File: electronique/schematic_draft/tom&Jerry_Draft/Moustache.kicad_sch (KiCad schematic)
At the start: 9 parts, among them IC3 IIM-20670, J4 Conn_01x08, J5 Conn_01x04, J6 Conn_01x04, J7 Conn_01x04, J8 Conn_01x04

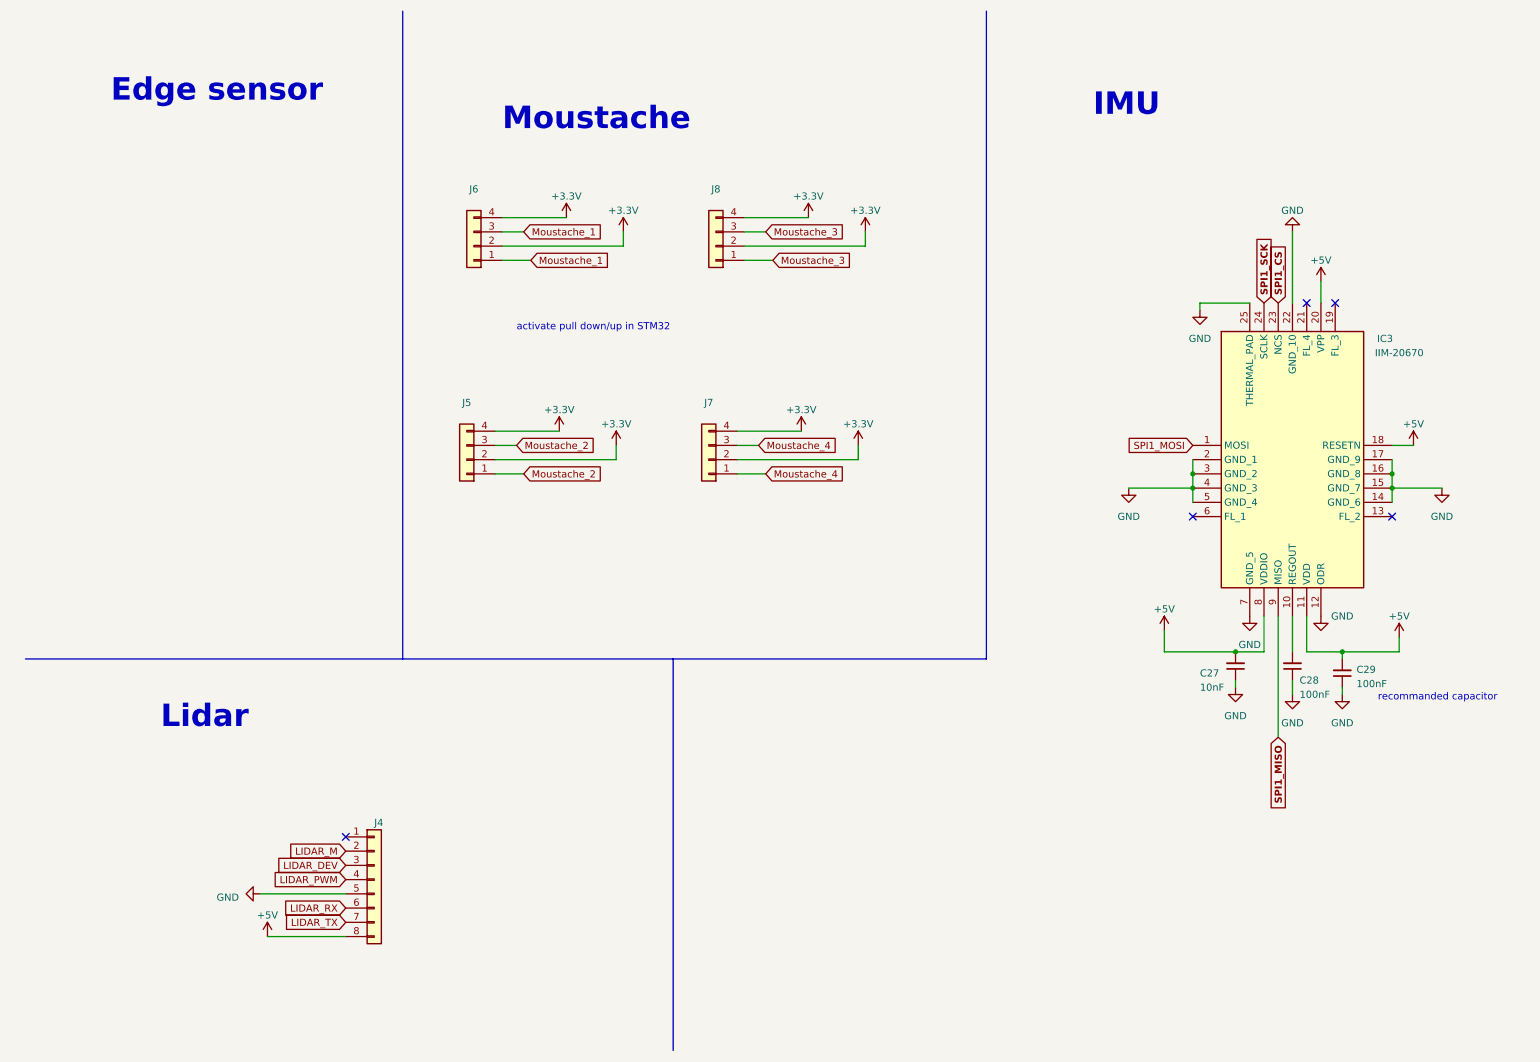
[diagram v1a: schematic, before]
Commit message: STM32 KiCAD V2 - 18.09.2024
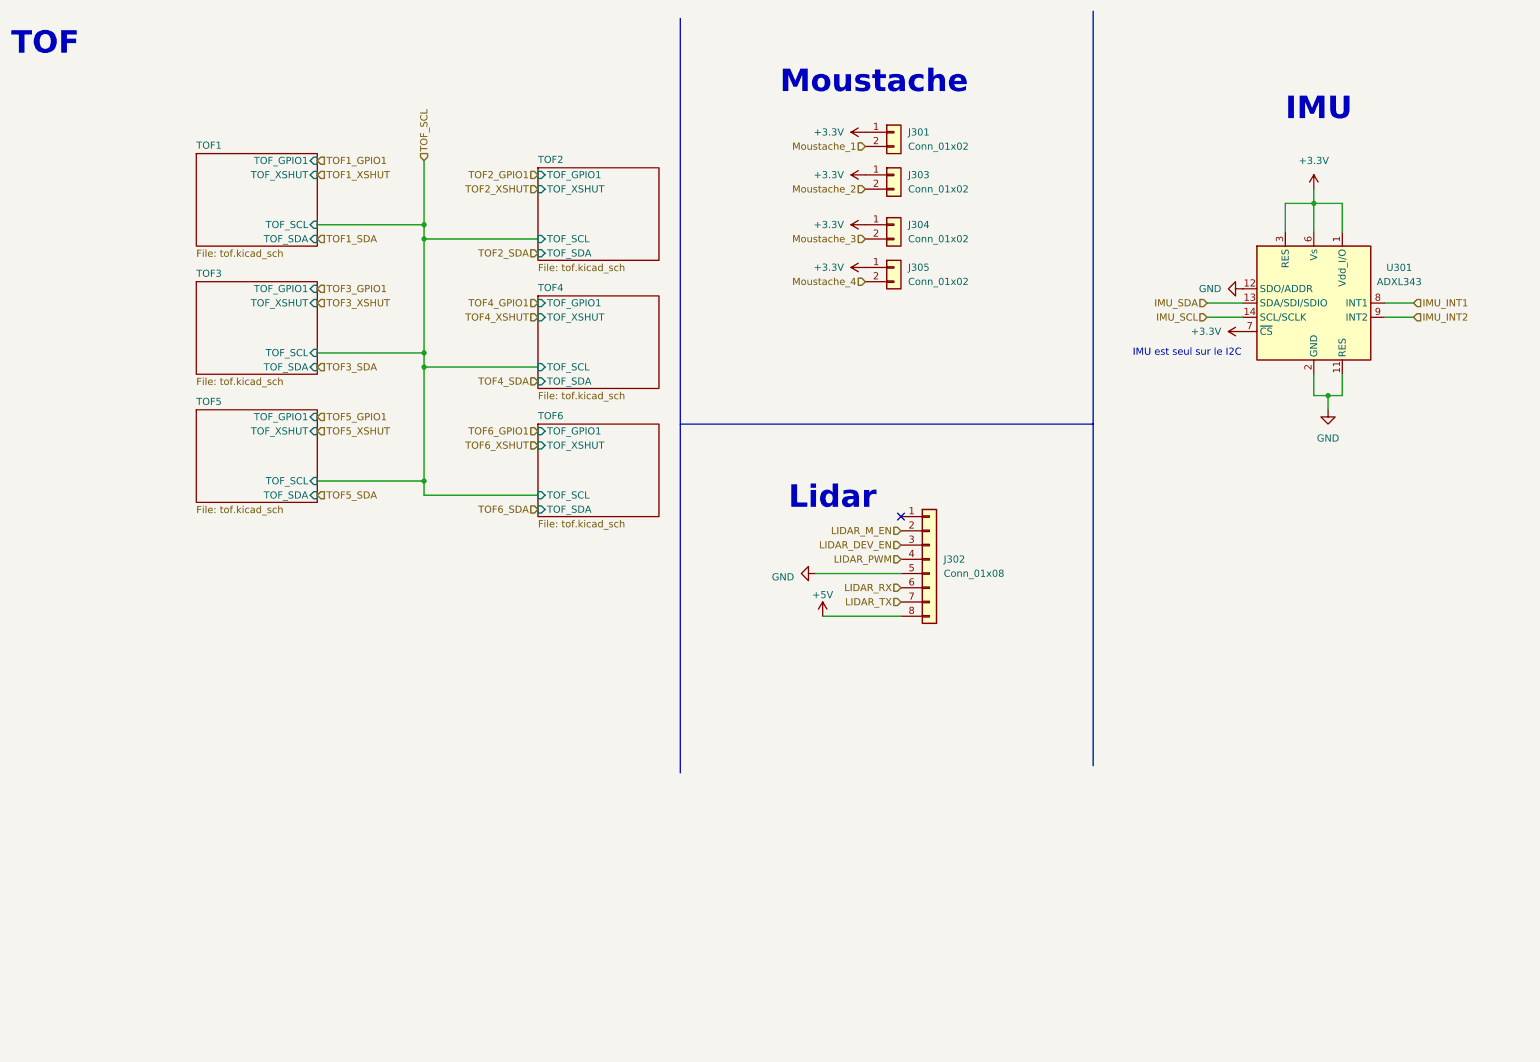
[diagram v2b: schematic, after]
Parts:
- removed C27: 10nF, Capacitor_SMD:C_0603_1608Metric_Pad1.08x0.95mm_HandSolder, symbol Device:C_Small
- removed C28, C29: 100nF, Capacitor_SMD:C_0603_1608Metric_Pad1.08x0.95mm_HandSolder, symbol Device:C_Small
- removed IC3: IIM-20670, Library:IMU, symbol Ludzlib:IIM-20670
- removed J4: Conn_01x08, Connector_JST:JST_XH_S8B-XH-A_1x08_P2.50mm_Horizontal, symbol Connector_Generic:Conn_01x08
- removed J5, J6, J7, J8: Conn_01x04, Connector_JST:JST_XH_S4B-XH-A_1x04_P2.50mm_Horizontal, symbol Connector_Generic:Conn_01x04
- added J301, J303, J304, J305: Conn_01x02, symbol Connector_Generic:Conn_01x02
- added J302: Conn_01x08, symbol Connector_Generic:Conn_01x08
- added U301: ADXL343, Package_LGA:LGA-14_3x5mm_P0.8mm_LayoutBorder1x6y, symbol Sensor_Motion:ADXL343
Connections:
- net +3.3V: now also J301.1 (Pin_1), J303.1 (Pin_1), J304.1 (Pin_1), J305.1 (Pin_1), U301.1 (Vdd_I/O), U301.3 (RES), U301.6 (Vs), U301.7 (~{CS})
- net +5V: now also J302.8 (Pin_8)
- net GND: now also J302.5 (Pin_5), U301.11 (RES), U301.12 (SDO/ADDR), U301.2 (GND), U301.4 (GND), U301.5 (GND)
- net LIDAR_PWM: now also J302.4 (Pin_4)
- net LIDAR_RX: now also J302.6 (Pin_6)
- net LIDAR_TX: now also J302.7 (Pin_7)
- net Moustache_1: now also J301.2 (Pin_2)
- net Moustache_2: now also J303.2 (Pin_2)
- net Moustache_3: now also J304.2 (Pin_2)
- net Moustache_4: now also J305.2 (Pin_2)
- new net IMU_INT1: U301.8 (INT1)
- new net IMU_INT2: U301.9 (INT2)
- new net IMU_SCL: U301.14 (SCL/SCLK)
- new net IMU_SDA: U301.13 (SDA/SDI/SDIO)
- new net LIDAR_DEV_EN: J302.3 (Pin_3)
- new net LIDAR_M_EN: J302.2 (Pin_2)
- no-connect marks 5 -> 1
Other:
- added sheet TOF1 (tof.kicad_sch)
- added sheet TOF2 (tof.kicad_sch)
- added sheet TOF3 (tof.kicad_sch)
- added sheet TOF4 (tof.kicad_sch)
- added sheet TOF5 (tof.kicad_sch)
- added sheet TOF6 (tof.kicad_sch)
- note added: "IMU est seul sur le I2C"
- note added: "TOF"
- note removed: "Edge sensor"
- note removed: "activate pull down/up in STM32"
- note removed: "recommanded capacitor"
